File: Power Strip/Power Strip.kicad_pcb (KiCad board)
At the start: 2 copper layers, 60.2 x 7.5 mm, 0 parts

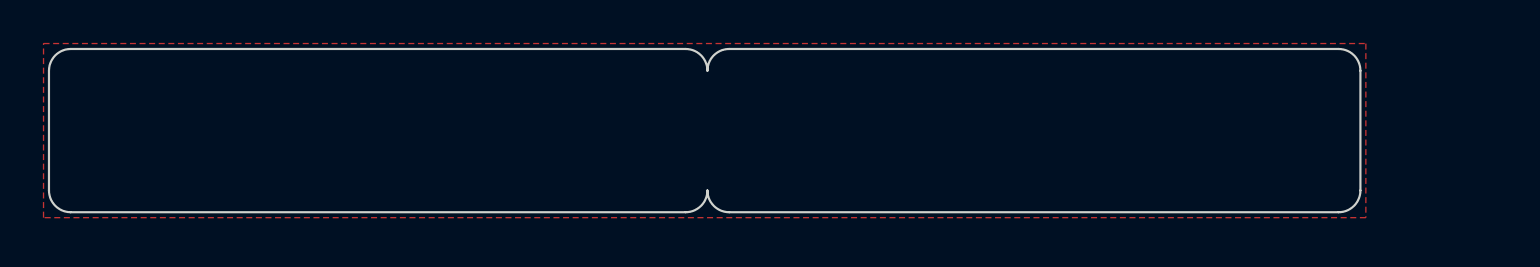
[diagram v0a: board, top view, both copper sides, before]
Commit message: updated files
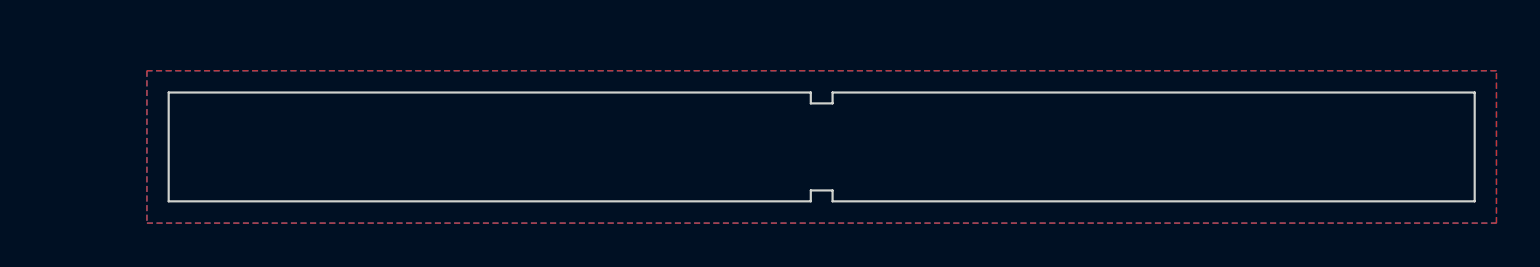
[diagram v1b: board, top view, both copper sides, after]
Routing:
- added copper zone on B.Cu, net (none)
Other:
- board size 60.2 x 7.5 mm -> 60 x 5 mm
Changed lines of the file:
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@@
-(kicad_pcb (version 20211014) (generator pcbnew)
+(kicad_pcb (version 20221018) (generator pcbnew)
   (general
     (thickness 1.6)
@@
     (pcbplotparams
       (layerselection 0x00010fc_ffffffff)
+      (plot_on_all_layers_selection 0x0000000_00000000)
       (disableapertmacros false)
       (usegerberextensions false)
@@
       (usegerberadvancedattributes true)
       (creategerberjobfile true)
-      (svguseinch false)
+      (dashed_line_dash_ratio 12.000000)
+      (dashed_line_gap_ratio 3.000000)
       (svgprecision 6)
-      (excludeedgelayer true)
       (plotframeref false)
       (viasonmask false)
@@
   )
   (net 0 "")
-  (gr_arc (start 145.75 106.5) (mid 145.042893 106.207107) (end 144.75 105.5) (layer "Edge.Cuts") (width 0.1))
-  (gr_arc (start 115.5 106.5) (mid 114.792893 106.207107) (end 114.5 105.5) (layer "Edge.Cuts") (width 0.1))
-  (gr_arc (start 174.75 105.5) (mid 174.457107 106.207107) (end 173.75 106.5) (layer "Edge.Cuts") (width 0.1))
-  (gr_arc (start 173.75 99) (mid 174.457107 99.292893) (end 174.75 100) (layer "Edge.Cuts") (width 0.1))
-  (gr_line (start 173.75 106.5) (end 145.75 106.5) (layer "Edge.Cuts") (width 0.1))
-  (gr_line (start 143.75 106.5) (end 115.5 106.5) (layer "Edge.Cuts") (width 0.1))
-  (gr_arc (start 144.75 100) (mid 145.042893 99.292893) (end 145.75 99) (layer "Edge.Cuts") (width 0.1))
-  (gr_arc (start 143.75 99) (mid 144.457107 99.292893) (end 144.75 100) (layer "Edge.Cuts") (width 0.1))
-  (gr_line (start 145.75 99) (end 173.75 99) (layer "Edge.Cuts") (width 0.1))
-  (gr_line (start 174.75 100) (end 174.75 105.5) (layer "Edge.Cuts") (width 0.1))
-  (gr_line (start 115.5 99) (end 143.75 99) (layer "Edge.Cuts") (width 0.1))
-  (gr_arc (start 144.75 105.5) (mid 144.457107 106.207107) (end 143.75 106.5) (layer "Edge.Cuts") (width 0.1))
-  (gr_line (start 114.5 105.5) (end 114.5 100) (layer "Edge.Cuts") (width 0.1))
-  (gr_arc (start 114.5 100) (mid 114.792893 99.292893) (end 115.5 99) (layer "Edge.Cuts") (width 0.1))
-  (zone (net 0) (net_name "") (layer "F.Cu") (hatch edge 0.508)
-    (connect_pads yes (clearance 0.5))
-    (min_thickness 0.127) (filled_areas_thickness no)
-    (fill yes (thermal_gap 0.127) (thermal_bridge_width 0.508) (island_removal_mode 1) (island_area_min 0))
+  (gr_line (start 149.5 101) (end 149.5 101.5)
+    (stroke (width 0.1) (type default)) (layer "Edge.Cuts"))
+  (gr_line (start 120 106) (end 120 101)
+    (stroke (width 0.1) (type default)) (layer "Edge.Cuts"))
+  (gr_line (start 150.5 101) (end 180 101)
+    (stroke (width 0.1) (type default)) (layer "Edge.Cuts"))
+  (gr_line (start 120 101) (end 149.5 101)
+    (stroke (width 0.1) (type default)) (layer "Edge.Cuts"))
+  (gr_line (start 149.5 105.5) (end 150.5 105.5)
+    (stroke (width 0.1) (type default)) (layer "Edge.Cuts"))
+  (gr_line (start 150.5 105.5) (end 150.5 106)
+    (stroke (width 0.1) (type default)) (layer "Edge.Cuts"))
+  (gr_line (start 149.5 101.5) (end 150.5 101.5)
+    (stroke (width 0.1) (type default)) (layer "Edge.Cuts"))
+  (gr_line (start 149.5 106) (end 149.5 105.5)
+    (stroke (width 0.1) (type default)) (layer "Edge.Cuts"))
+  (gr_line (start 149.5 106) (end 120 106)
+    (stroke (width 0.1) (type default)) (layer "Edge.Cuts"))
+  (gr_line (start 180 101) (end 180 106)
+    (stroke (width 0.1) (type default)) (layer "Edge.Cuts"))
+  (gr_line (start 150.5 101.5) (end 150.5 101)
+    (stroke (width 0.1) (type default)) (layer "Edge.Cuts"))
+  (gr_line (start 180 106) (end 150.5 106)
+    (stroke (width 0.1) (type default)) (layer "Edge.Cuts"))
+  (zone (net 0) (net_name "") (layers "F&B.Cu") (hatch edge 0.5)
+    (connect_pads (clearance 0.5))
+    (min_thickness 0.25) (filled_areas_thickness no)
+    (fill yes (thermal_gap 0.5) (thermal_bridge_width 0.5) (island_removal_mode 1) (island_area_min 10))
     (polygon
       (pts
-        (xy 175 106.75)
-        (xy 114.25 106.75)
-        (xy 114.25 98.75)
-        (xy 175 98.75)
+        (xy 119 100)
+        (xy 119 107)
+        (xy 181 107)
+        (xy 181 100)
       )
     )
   )
-  (zone (net 0) (net_name "") (layers *.Mask) (hatch edge 0.508)
-    (connect_pads yes (clearance 0.5))
-    (min_thickness 0.127) (filled_areas_thickness no)
-    (fill yes (thermal_gap 0.127) (thermal_bridge_width 0.508) (island_removal_mode 1) (island_area_min 0))
+  (zone (net 0) (net_name "") (layers "*.Mask") (hatch edge 0.5)
+    (connect_pads (clearance 0.5))
+    (min_thickness 0.25) (filled_areas_thickness no)
+    (fill yes (thermal_gap 0.5) (thermal_bridge_width 0.5))
     (polygon
       (pts
-        (xy 175.25 107)
-        (xy 114 107)
-        (xy 114 98.5)
-        (xy 175.25 98.5)
+        (xy 118 99)
+        (xy 118 108)
+        (xy 182 108)
+        (xy 182 99)
       )
     )
